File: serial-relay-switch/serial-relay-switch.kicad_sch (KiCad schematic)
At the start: 79 parts, among them J1 Screw_Terminal_01x01, J10 Screw_Terminal_01x01, J11 Screw_Terminal_01x01, J15 Screw_Terminal_01x01, J16 Screw_Terminal_01x01, J17 Conn_01x01, J18 Conn_01x01, J19 Screw_Terminal_01x01, J2 2501551-4, J20 Screw_Terminal_01x01, J21 Conn_01x01, J4 Screw_Terminal_01x01, J5 Screw_Terminal_01x01, J6 Screw_Terminal_01x01, J7 Screw_Terminal_01x01, J8 Screw_Terminal_01x01, J9 Screw_Terminal_01x01, K1 G2RL-1-E, K2 G2RL-1-E, K3 G2RL-1-E, K4 G2RL-1-E, K5 G2RL-1-E, K6 G2RL-1-E, K7 G2RL-1-E, K8 G2RL-1-E, U1 H11L1, U10 SZNUD3124LT1G, U11 SZNUD3124LT1G, U12 SZNUD3124LT1G, U13 74HCT595, U14 74LVC1G32, U15 74LVC1G08, U16 74LVC1G04, U17 74LS163, U2 ISL8488E, U3 SZNUD3124LT1G, U4 ISL8488E, U6 SZNUD3124LT1G, U7 SZNUD3124LT1G, U8 SZNUD3124LT1G, U9 SZNUD3124LT1G

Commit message: [rs] Footprint assignment
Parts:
- D1: footprint (none) -> Diode_SMD:D_SOD-123F
- D2, D3, D4, D5, D6, D7, D8, D9: footprint (none) -> LED_SMD:LED_0603_1608Metric
- R1, R2, R3, R4, R5, R6, R7, R8: footprint (none) -> Resistor_SMD:R_0603_1608Metric
- U14, U15, U16: footprint (none) -> Package_TO_SOT_SMD:SOT-23-5
- U17: footprint (none) -> Package_SO:SOIC-16_3.9x9.9mm_P1.27mm
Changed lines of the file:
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@@
 			)
 		)
-		(property "Footprint" ""
+		(property "Footprint" "Package_SO:SOIC-16_3.9x9.9mm_P1.27mm"
 			(at 63.5 134.62 0)
 			(hide yes)
@@
 			)
 		)
-		(property "Footprint" ""
+		(property "Footprint" "LED_SMD:LED_0603_1608Metric"
 			(at 297.18 154.94 0)
 			(hide yes)
@@
 			)
 		)
-		(property "Footprint" ""
+		(property "Footprint" "LED_SMD:LED_0603_1608Metric"
 			(at 276.86 203.2 0)
 			(hide yes)
@@
 			)
 		)
-		(property "Footprint" ""
+		(property "Footprint" "Diode_SMD:D_SOD-123F"
 			(at 50.8 58.42 0)
 			(hide yes)
@@
 			)
 		)
-		(property "Footprint" ""
+		(property "Footprint" "Package_TO_SOT_SMD:SOT-23-5"
 			(at 154.94 152.4 0)
 			(hide yes)
@@
 			)
 		)
-		(property "Footprint" ""
+		(property "Footprint" "LED_SMD:LED_0603_1608Metric"
 			(at 297.18 58.42 0)
 			(hide yes)
@@
 			)
 		)
-		(property "Footprint" ""
+		(property "Footprint" "Resistor_SMD:R_0603_1608Metric"
 			(at 284.48 60.198 90)
 			(hide yes)
@@
 			)
 		)
-		(property "Footprint" ""
+		(property "Footprint" "LED_SMD:LED_0603_1608Metric"
 			(at 297.18 106.68 0)
 			(hide yes)
@@
 			)
 		)
-		(property "Footprint" ""
+		(property "Footprint" "Resistor_SMD:R_0603_1608Metric"
 			(at 347.98 204.978 90)
 			(hide yes)
@@
 			)
 		)
-		(property "Footprint" ""
+		(property "Footprint" "Resistor_SMD:R_0603_1608Metric"
 			(at 347.98 60.198 90)
 			(hide yes)
@@
 			)
 		)
-		(property "Footprint" ""
+		(property "Footprint" "Resistor_SMD:R_0603_1608Metric"
 			(at 284.48 156.718 90)
 			(hide yes)
@@
 			)
 		)
-		(property "Footprint" ""
+		(property "Footprint" "Package_TO_SOT_SMD:SOT-23-5"
 			(at 109.22 109.22 0)
 			(hide yes)
@@
 			)
 		)
-		(property "Footprint" ""
+		(property "Footprint" "Resistor_SMD:R_0603_1608Metric"
 			(at 347.98 156.718 90)
 			(hide yes)
@@
 			)
 		)
-		(property "Footprint" ""
+		(property "Footprint" "Resistor_SMD:R_0603_1608Metric"
 			(at 284.48 108.458 90)
 			(hide yes)
@@
 			)
 		)
-		(property "Footprint" ""
+		(property "Footprint" "LED_SMD:LED_0603_1608Metric"
 			(at 360.68 154.94 0)
 			(hide yes)
@@
 			)
 		)
-		(property "Footprint" ""
+		(property "Footprint" "Resistor_SMD:R_0603_1608Metric"
 			(at 347.98 108.458 90)
 			(hide yes)
@@
 			)
 		)
-		(property "Footprint" ""
+		(property "Footprint" "LED_SMD:LED_0603_1608Metric"
 			(at 360.68 58.42 0)
 			(hide yes)
@@
 			)
 		)
-		(property "Footprint" ""
+		(property "Footprint" "LED_SMD:LED_0603_1608Metric"
 			(at 360.68 203.2 0)
 			(hide yes)
@@
 			)
 		)
-		(property "Footprint" ""
+		(property "Footprint" "Package_TO_SOT_SMD:SOT-23-5"
 			(at 154.94 111.76 0)
 			(hide yes)
@@
 			)
 		)
-		(property "Footprint" ""
+		(property "Footprint" "LED_SMD:LED_0603_1608Metric"
 			(at 360.68 106.68 0)
 			(hide yes)
@@
 			)
 		)
-		(property "Footprint" ""
+		(property "Footprint" "Resistor_SMD:R_0603_1608Metric"
 			(at 264.16 204.978 90)
 			(hide yes)

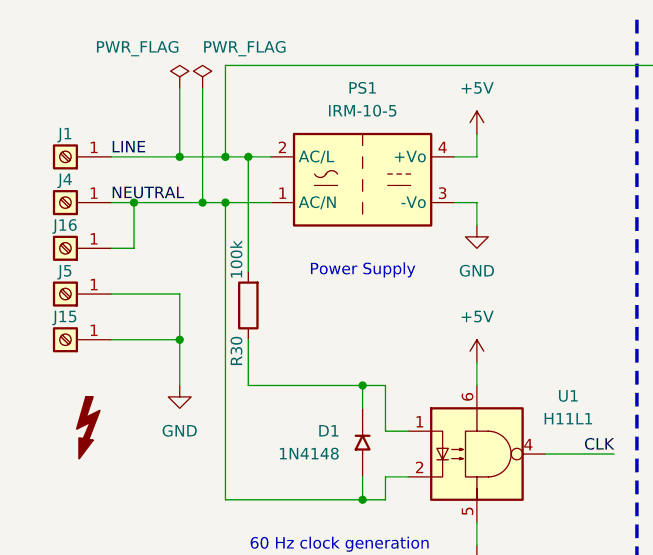
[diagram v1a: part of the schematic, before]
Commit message: [rs] Mostly complete preliminary PCB placement
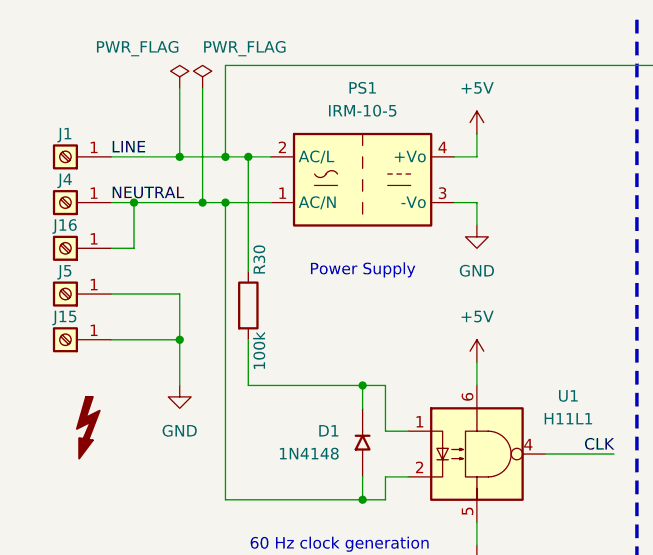
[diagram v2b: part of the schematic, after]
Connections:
- net LINE: now also R30.1; no longer R30.2
- net at D1.1 (K), U1.1: now also R30.2; no longer R30.1
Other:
- moved on the sheet: R30
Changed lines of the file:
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@@
 	)
 	(junction
+		(at 38.1 27.94)
+		(diameter 0)
+		(color 0 0 0 0)
+	)
+	(junction
 		(at 340.36 198.12)
 		(diameter 0)
@@
 	)
 	(junction
-		(at 38.1 27.94)
-		(diameter 0)
-		(color 0 0 0 0)
-	)
-	(junction
 		(at 101.6 228.6)
 		(diameter 0)
@@
 	(wire
 		(pts
-			(xy 38.1 53.34) (xy 38.1 48.26)
-		)
-		(stroke
-			(width 0)
-			(type default)
-		)
-	)
-	(wire
-		(pts
 			(xy 35.56 33.02) (xy 40.64 33.02)
 		)
@@
 	(wire
 		(pts
-			(xy 35.56 27.94) (xy 40.64 27.94)
+			(xy 35.56 27.94) (xy 38.1 27.94)
 		)
 		(stroke
@@
 	(wire
 		(pts
-			(xy 38.1 40.64) (xy 38.1 27.94)
+			(xy 38.1 27.94) (xy 38.1 40.64)
 		)
 		(stroke
@@
 	(wire
 		(pts
+			(xy 38.1 48.26) (xy 38.1 53.34)
+		)
+		(stroke
+			(width 0)
+			(type default)
+		)
+	)
+	(wire
+		(pts
 			(xy 391.16 17.78) (xy 327.66 17.78)
 		)
@@
 	(wire
 		(pts
+			(xy 38.1 27.94) (xy 40.64 27.94)
+		)
+		(stroke
+			(width 0)
+			(type default)
+		)
+	)
+	(wire
+		(pts
 			(xy 317.5 96.52) (xy 327.66 96.52)
 		)
@@
 	(symbol
 		(lib_id "CUSTOM:R")
-		(at 38.1 45.72 180)
+		(at 38.1 43.18 0)
 		(unit 1)
 		(body_style 1)
@@
 		(dnp no)
 		(property "Reference" "R30"
-			(at 36.83 49.53 90)
+			(at 39.37 39.37 90)
 			(show_name no)
 			(do_not_autoplace no)
@@
 		)
 		(property "Value" "100k"
-			(at 36.83 39.37 90)
+			(at 39.37 49.53 90)
 			(show_name no)
 			(do_not_autoplace no)
@@
 		)
 		(property "Footprint" "Resistor_THT:R_Axial_DIN0414_L11.9mm_D4.5mm_P5.08mm_Vertical"
-			(at 39.878 45.72 90)
+			(at 36.322 43.18 90)
 			(hide yes)
 			(show_name no)
@@
 		)
 		(property "Datasheet" ""
-			(at 38.1 45.72 0)
+			(at 38.1 43.18 0)
 			(hide yes)
 			(show_name no)
